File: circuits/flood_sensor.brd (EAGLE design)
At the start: 81 x 81 mm, 52 parts, among them T1 BC847, U1 MMA8452Q, U2 LM1117, U3 DS18B20, U5 LMV358M

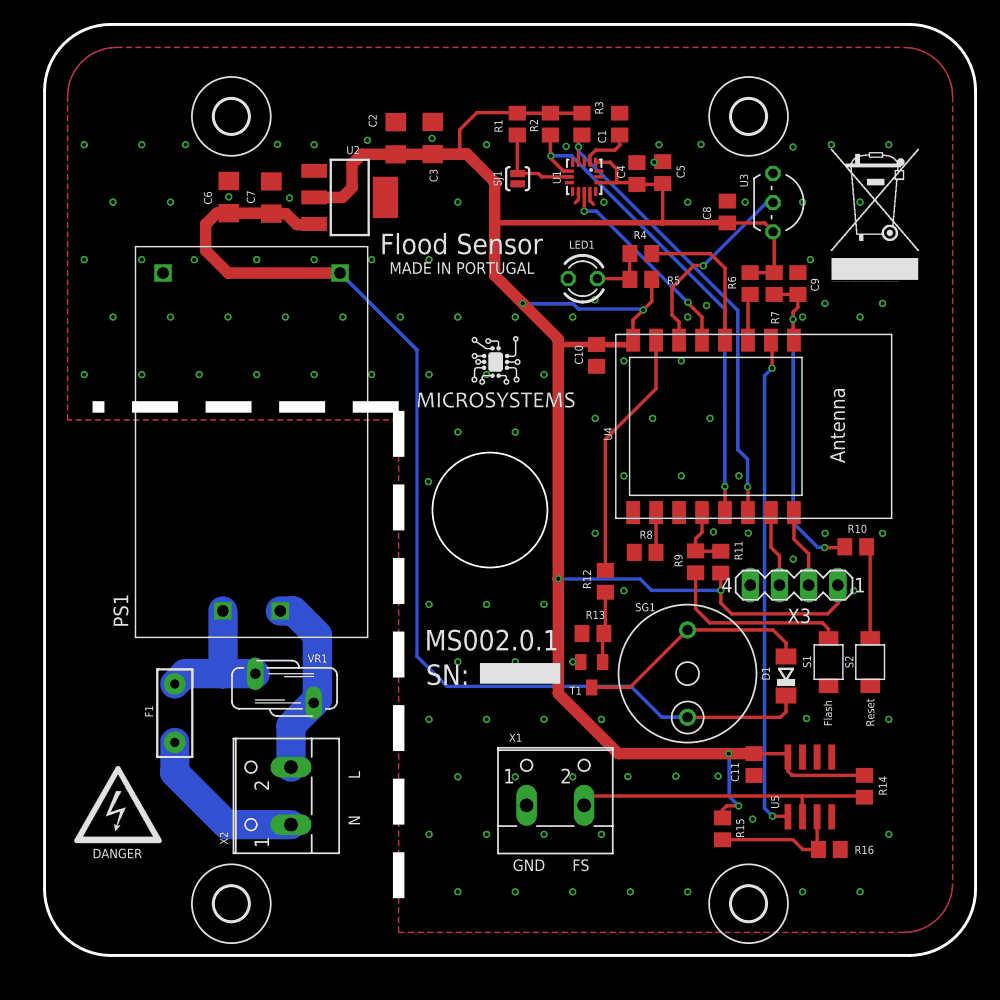
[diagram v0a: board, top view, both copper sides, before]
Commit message: finished first revision
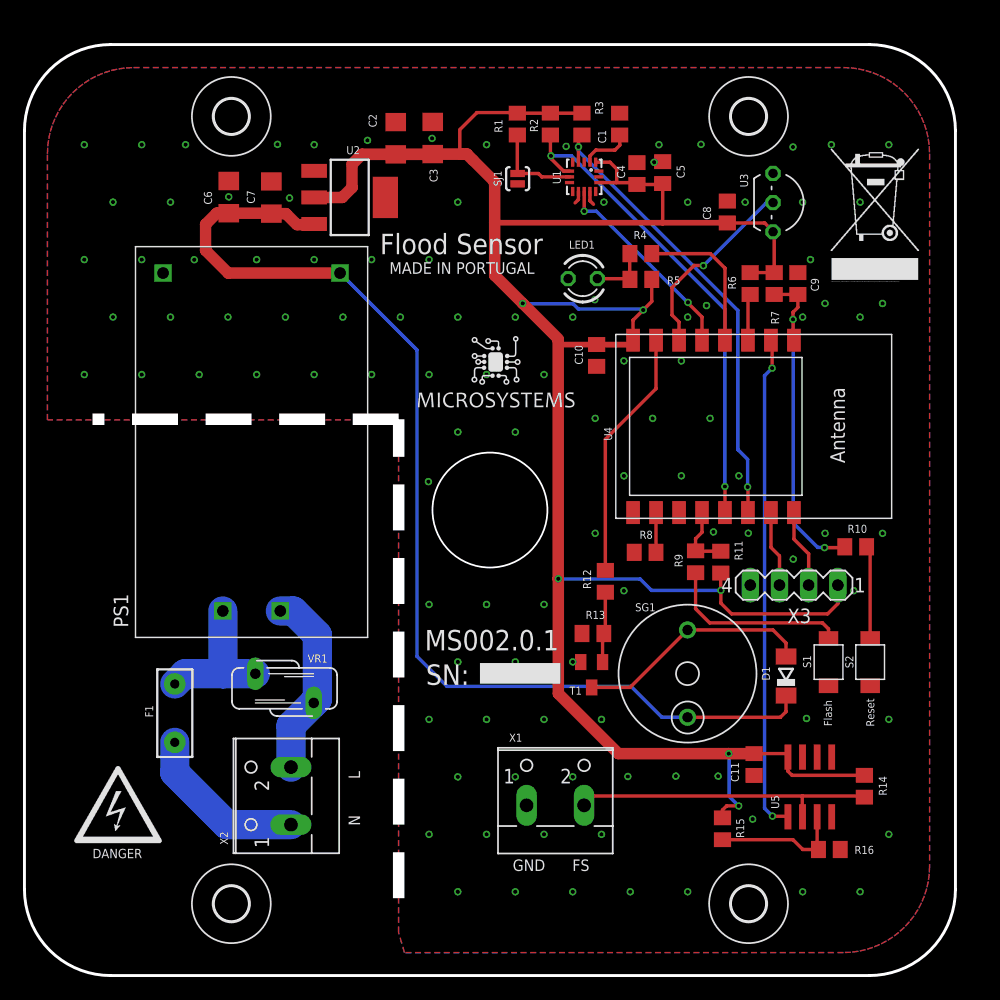
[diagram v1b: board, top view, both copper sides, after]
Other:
- outline, holes or cut-outs redrawn
